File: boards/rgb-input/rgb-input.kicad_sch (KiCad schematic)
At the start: 7 parts, among them J42 INPUTS, U1 ESP32-DEVKITC

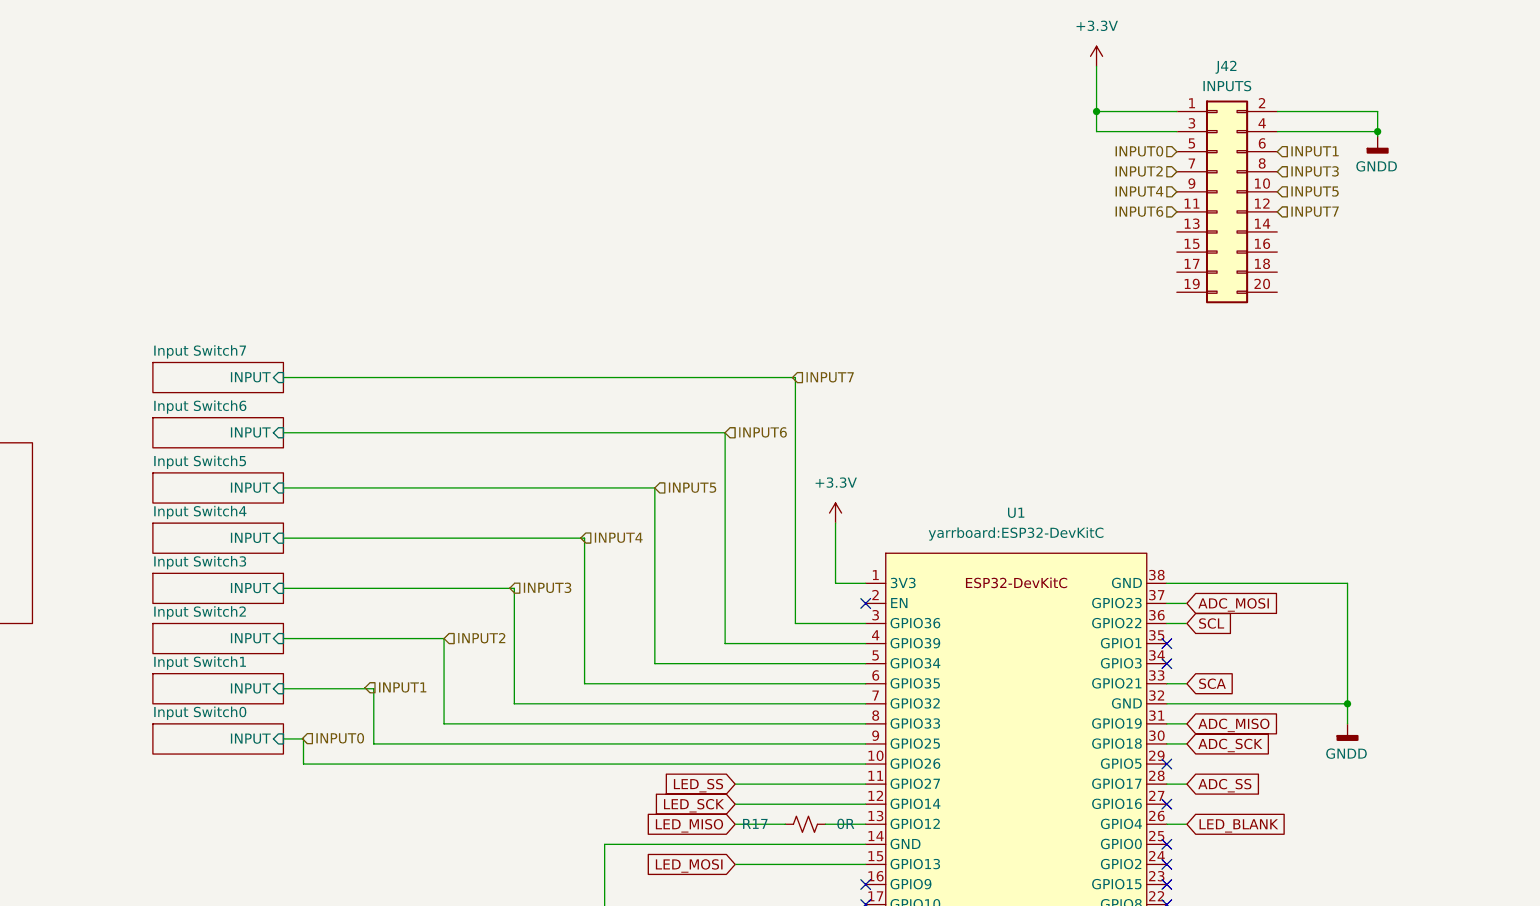
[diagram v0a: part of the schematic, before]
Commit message: new rgb input board coming along very nicely
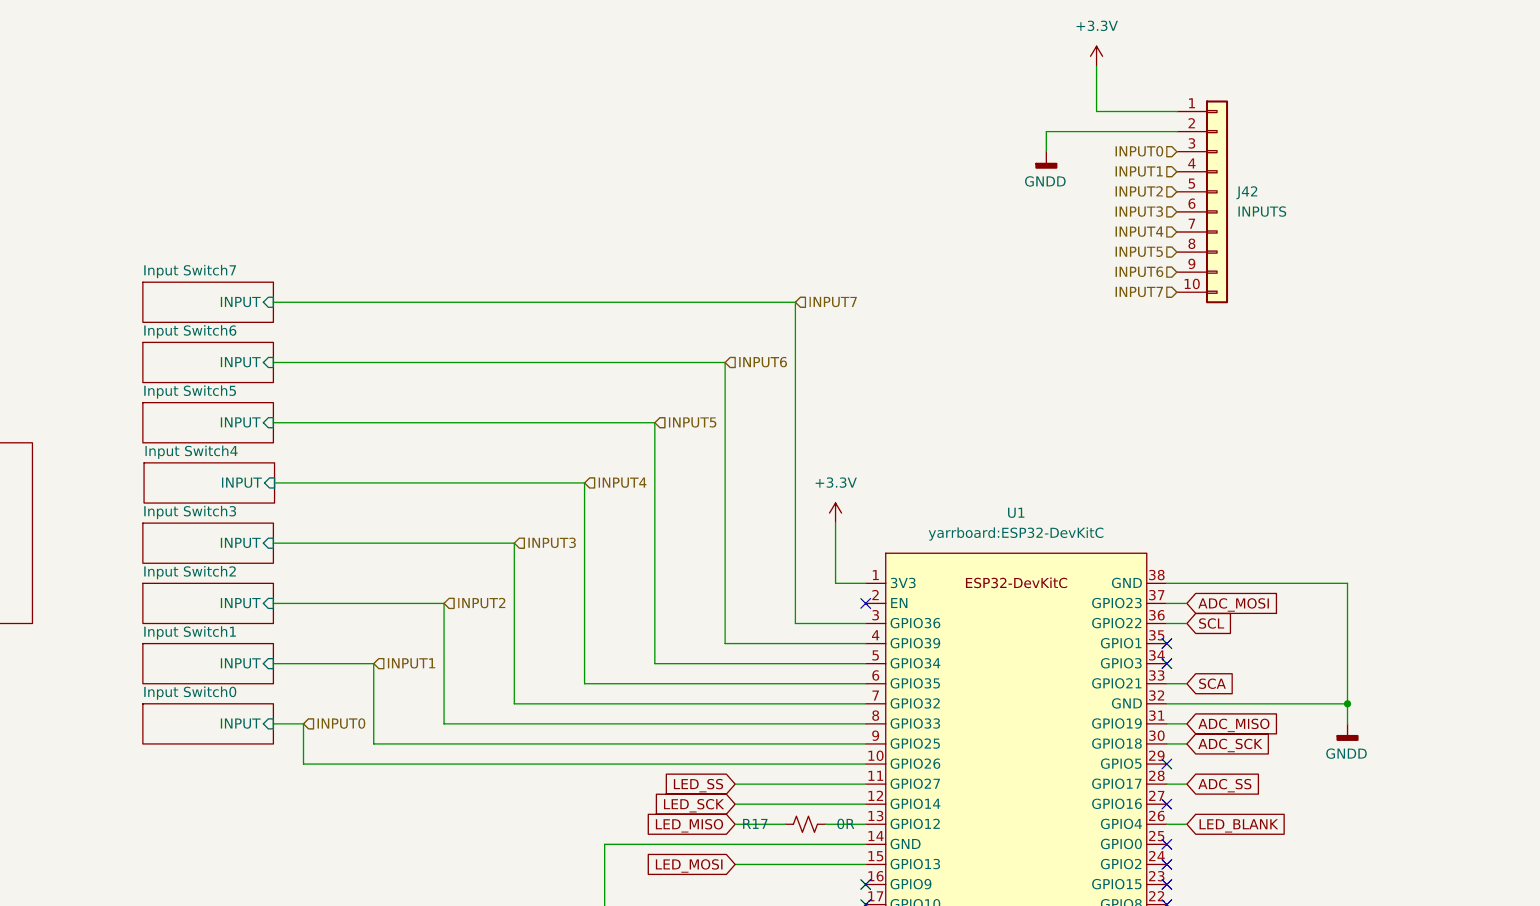
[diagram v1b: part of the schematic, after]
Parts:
- J42: footprint Connector_IDC:IDC-Header_2x10_P2.54mm_Vertical -> Connector_FFC-FPC:Molex_200528-0100_1x10-1MP_P1.00mm_Horizontal; symbol Connector_Generic:Conn_02x10_Odd_Even -> Connector_Generic:Conn_01x10
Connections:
- net Input Switch0/INPUT is gone; now on net INPUT0: U1.10 (GPIO26)
- net Input Switch1/INPUT is gone; now on net INPUT1: U1.9 (GPIO25)
- net Input Switch3/INPUT is gone; now on net INPUT3: U1.7 (GPIO32)
- net Input Switch4/INPUT is gone; now on net INPUT4: U1.6 (GPIO35)
- net Input Switch7/INPUT is gone; now on net INPUT7: U1.3 (GPIO36)
- net +3.3V: no longer J42.3 (Pin_3)
- net GNDD: no longer J42.4 (Pin_4)
- net INPUT0: now also J42.3 (Pin_3); no longer J42.5 (Pin_5)
- net INPUT1: now also J42.4 (Pin_4); no longer J42.6 (Pin_6)
- net INPUT2: now also J42.5 (Pin_5); no longer J42.7 (Pin_7)
- net INPUT3: now also J42.6 (Pin_6); no longer J42.8 (Pin_8)
- net INPUT4: now also J42.7 (Pin_7); no longer J42.9 (Pin_9)
- net INPUT5: now also J42.8 (Pin_8); no longer J42.10 (Pin_10)
- net INPUT6: now also J42.9 (Pin_9); no longer J42.11 (Pin_11)
- net INPUT7: now also J42.10 (Pin_10); no longer J42.12 (Pin_12)
